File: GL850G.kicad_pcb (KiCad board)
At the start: 4 copper layers, 75 x 55 mm, 52 parts, among them J1 USB_A, J10 Conn_01x02_Pin, J2 USB_A, J3 USB_A, J4 USB_A, J5 USB_A, J6 Conn_01x03_Pin, J7 Conn_01x02_Pin, J8 Conn_01x02_Pin, J9 Conn_01x03_Pin, U1 GL850G, U11 AP2151WG, Y1 12MHz

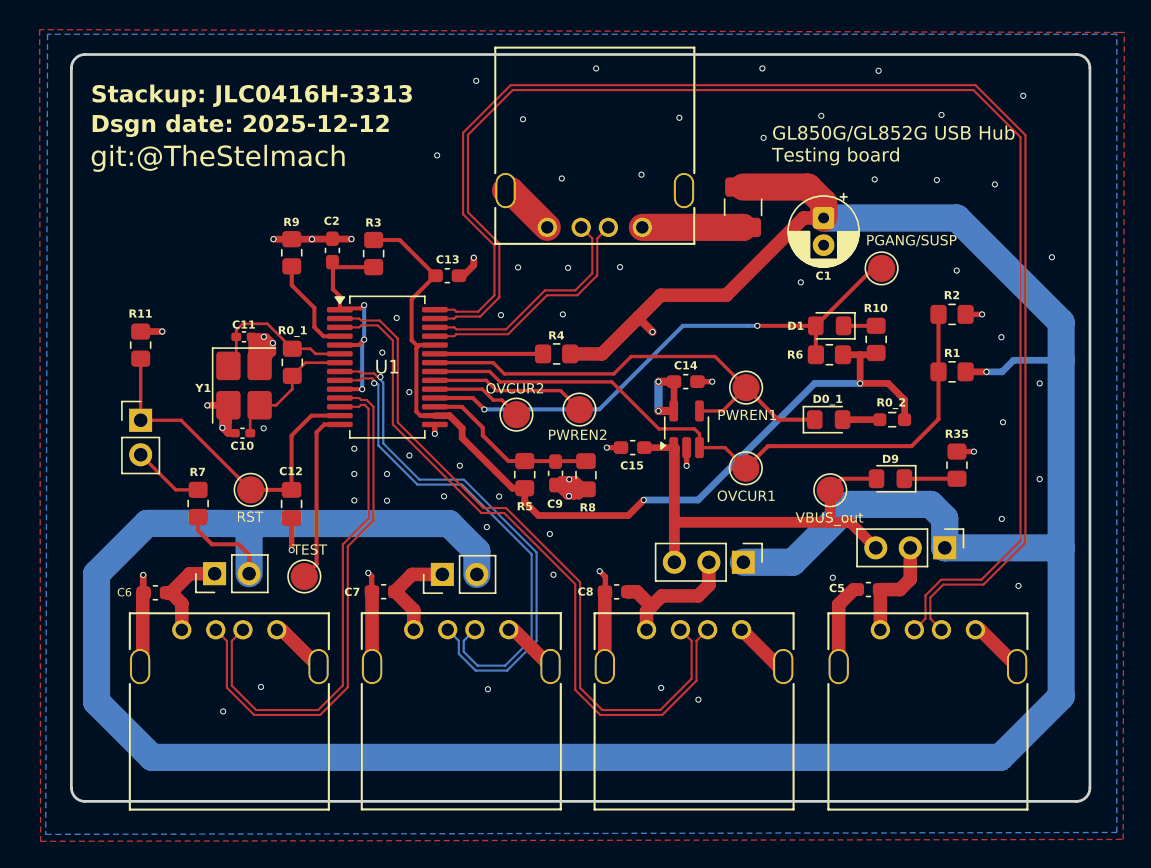
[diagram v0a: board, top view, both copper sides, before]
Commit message: modified:   0.My_Library.bak 	modified:   0.My_Library.kicad_sym 	new file:   GL850G-backups/GL850G-2026-01-02_150657.zip 	new file:   GL850G-backups/GL850G-2026-01-02_151627.zip 	new file:   GL850G-backups/GL850G-2026-01-02_160446.zip 	new file:   GL850G-backups/GL850G-2026-01-03_192335.zip 	new file:   GL850G-backups/GL850G-2026-01-03_193700.zip 	new file:   GL850G-backups/GL850G-2026-01-03_194723.zip 	new file:   GL850G-backups/GL850G-2026-01-03_195234.zip 	new file:   GL850G-backups/GL850G-2026-01-03_195824.zip 	modified:   GL850G.kicad_pcb 	modified:   GL850G.kicad_pro 	modified:   GL850G.kicad_sch 	new file:   GL850G_USB_Hub_BACKUP.zip 	modified:   fp-info-cache 	modified:   production/GL850G.zip 	new file:   production/backups/GL850G_2026-01-03_19-52-49.zip 	modified:   production/bom.csv 	modified:   production/designators.csv 	modified:   production/netlist.ipc 	modified:   production/positions.csv
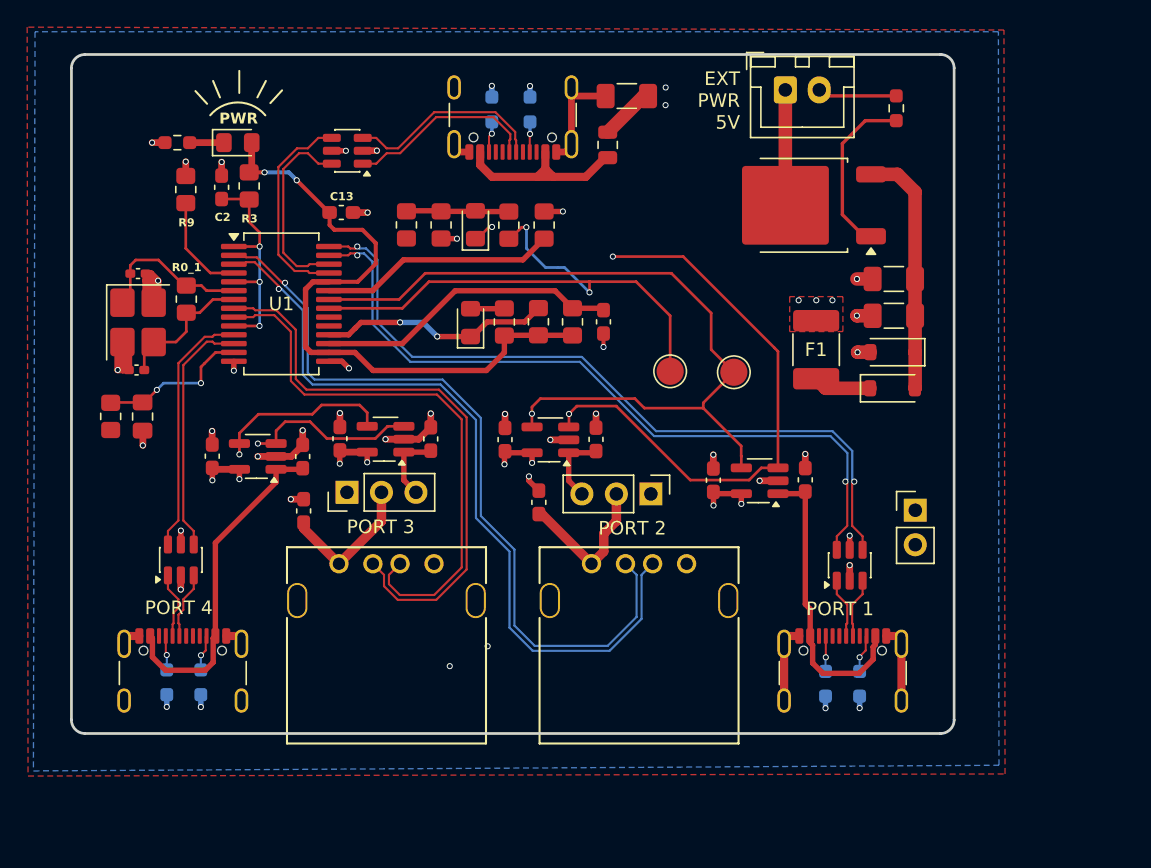
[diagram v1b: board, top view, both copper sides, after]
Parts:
- removed D9: LED, LED_SMD:LED_0805_2012Metric_Pad1.15x1.40mm_HandSolder
- removed J10, J7, J8: Conn_01x02_Pin, Connector_PinHeader_2.54mm:PinHeader_1x02_P2.54mm_Vertical
- removed J6: Conn_01x03_Pin, Connector_PinHeader_2.54mm:PinHeader_1x03_P2.54mm_Vertical
- removed R11: 100k, Resistor_SMD:R_0805_2012Metric_Pad1.20x1.40mm_HandSolder
- removed R35: 500, Resistor_SMD:R_0805_2012Metric_Pad1.20x1.40mm_HandSolder
- removed TP1, TP3, TP4, TP6, TP7, TP8: TestPoint, TestPoint:TestPoint_Pad_D2.0mm
- added C16: 2.2uF, Capacitor_SMD:C_0603_1608Metric_Pad1.08x0.95mm_HandSolder, F.Cu at (140.8, 91.8)
- added C17: 2.2uF, Capacitor_SMD:C_0603_1608Metric_Pad1.08x0.95mm_HandSolder, F.Cu at (134.1, 91.8)
- added C18: 2.2uF, Capacitor_SMD:C_0603_1608Metric_Pad1.08x0.95mm_HandSolder, F.Cu at (131.3, 93.1)
- added C19: 2.2uF, Capacitor_SMD:C_0603_1608Metric_Pad1.08x0.95mm_HandSolder, F.Cu at (124.7, 93.1)
- added C3: 2.2uF, Capacitor_SMD:C_0603_1608Metric_Pad1.08x0.95mm_HandSolder, F.Cu at (152.9, 91.8)
- added C4: 2.2uF, Capacitor_SMD:C_0603_1608Metric_Pad1.08x0.95mm_HandSolder, F.Cu at (146.2, 91.9)
- added D2: LED, LED_SMD:LED_0805_2012Metric_Pad1.15x1.40mm_HandSolder, F.Cu at (144.1, 76.0)
- added D7: BZT52C5V6, Diode_SMD:D_SOD-123, F.Cu at (174.8, 85.4)
- added D8: B5819W, Diode_SMD:D_SOD-123, F.Cu at (174.8, 88.1)
- added F4: 500mA, Fuse:Fuse_0805_2012Metric, F.Cu at (153.8, 70.2)
- added Q1: 40p04, Package_TO_SOT_SMD:TO-252-2, F.Cu at (168.1, 74.6)
- added R13: 5.1k_1%, Resistor_SMD:R_0603_1608Metric_Pad0.98x0.95mm_HandSolder, B.Cu at (172.3, 109.8)
- added R14: 5.1k_1%, Resistor_SMD:R_0603_1608Metric_Pad0.98x0.95mm_HandSolder, B.Cu at (169.8, 109.8)
- added R15: 5.1k_1%, Resistor_SMD:R_0603_1608Metric_Pad0.98x0.95mm_HandSolder, B.Cu at (123.8, 109.7)
- added R16: 5.1k_1%, Resistor_SMD:R_0603_1608Metric_Pad0.98x0.95mm_HandSolder, B.Cu at (121.3, 109.7)
- added R26: 10k, Resistor_SMD:R_0603_1608Metric_Pad0.98x0.95mm_HandSolder, F.Cu at (175.0, 67.5)
- added R67: 5.1k_1%, Resistor_SMD:R_0603_1608Metric_Pad0.98x0.95mm_HandSolder, B.Cu at (145.3, 67.5)
- added R68: 5.1k_1%, Resistor_SMD:R_0603_1608Metric_Pad0.98x0.95mm_HandSolder, B.Cu at (148.1, 67.5)
- added U12: USBLC6-2SC6, Package_TO_SOT_SMD:SOT-23-6, F.Cu at (134.6, 70.6)
- added U2: AP2141WG, Package_TO_SOT_SMD:SOT-23-5_HandSoldering, F.Cu at (149.6, 91.9)
- added U3: AP2141WG, Package_TO_SOT_SMD:SOT-23-5_HandSoldering, F.Cu at (137.4, 91.8)
- added U4: AP2141WG, Package_TO_SOT_SMD:SOT-23-5_HandSoldering, F.Cu at (128.0, 93.1)
- added U5: USBLC6-2SC6, Package_TO_SOT_SMD:SOT-23-6, F.Cu at (171.6, 101.1)
- added U6: USBLC6-2SC6, Package_TO_SOT_SMD:SOT-23-6, F.Cu at (122.4, 100.7)
- added USB1: USB_C_Recep._USB2.0_16P, Connector_USB:USB_C_Receptacle_GCT_USB4105-xx-A_16P_TopMnt_Horizontal, F.Cu at (146.8, 67.0)
- added USB2: USB_C_Recep._USB2.0_16P, Connector_USB:USB_C_Receptacle_GCT_USB4105-xx-A_16P_TopMnt_Horizontal, F.Cu at (171.1, 110.0)
- added USB3: USB_C_Recep._USB2.0_16P, Connector_USB:USB_C_Receptacle_GCT_USB4105-xx-A_16P_TopMnt_Horizontal, F.Cu at (122.5, 110.0)
- C1: footprint Capacitor_THT:CP_Radial_D5.0mm_P2.00mm -> Capacitor_SMD:C_1206_3216Metric_Pad1.33x1.80mm_HandSolder
- C5, C6: value 100nF -> 100uF; footprint Capacitor_SMD:C_0603_1608Metric_Pad1.08x0.95mm_HandSolder -> Capacitor_SMD:C_1206_3216Metric_Pad1.33x1.80mm_HandSolder
- F1: value Fuse_Small -> Fuse; footprint Fuse:Fuse_1210_3225Metric_Pad1.42x2.65mm_HandSolder -> Capacitor_SMD:C_1812_4532Metric_Pad1.57x3.40mm_HandSolder
- J1: value USB_A -> Conn_01x03_Pin; footprint My_Library:USB_A_2.0 -> Connector_PinHeader_2.54mm:PinHeader_1x03_P2.54mm_Vertical
- J2: value USB_A -> 5V; footprint My_Library:USB_A_2.0 -> Connector_JST:JST_XH_B2B-XH-A_1x02_P2.50mm_Vertical
- J3: value USB_A -> 5V_OUT; footprint My_Library:USB_A_2.0 -> Connector_PinHeader_2.54mm:PinHeader_1x02_P2.54mm_Vertical
- R0_2: value 100k -> 1k
- R1: value 10k -> 1k
- R10: value 1k -> 2k
- R2: value 20k -> 2k
- R8: value ? -> 1k; footprint Capacitor_SMD:C_0805_2012Metric_Pad1.18x1.45mm_HandSolder -> Resistor_SMD:R_0805_2012Metric_Pad1.20x1.40mm_HandSolder
- U1: value GL850G -> GL850G/GL852G
- U11: value AP2151WG -> AP2141WG
- moved C6 59.1 mm to (174.9, 80.0)
- moved R0_2 56.5 mm to (122.1, 70.0)
- moved J3 51.3 mm to (176.4, 97.1)
- moved D0_1 48.1 mm to (126.6, 70.0)
- moved R1 41.6 mm to (139.0, 76.0), turned to -90 degrees
- moved J2 41.1 mm to (166.9, 66.1)
- moved R2 38.2 mm to (141.5, 76.1), turned to 90 degrees
- moved R10 27.4 mm to (146.2, 83.2), turned to 90 degrees
- moved J1 26.7 mm to (134.6, 95.7), turned to 90 degrees
- moved D1 26.4 mm to (143.7, 83.2), turned to 90 degrees
- moved R6 21.6 mm to (148.7, 83.2), turned to 90 degrees
- moved C5 20.2 mm to (174.9, 82.7), turned to 180 degrees
- moved R8 19.3 mm to (146.5, 76.1), turned to 90 degrees
- moved C1 17.0 mm to (155.2, 66.6), turned to 180 degrees
- moved C15 12.9 mm to (168.3, 94.8), turned to 90 degrees
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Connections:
- C15 pad 1: VBUS_out -> VBUS_out1
- C5 pad 1: Net-(J2-VBUS) -> Net-(D7-K)
- C6 pad 1: Net-(J3-VBUS) -> Net-(D7-K)
- C7 pad 1: Net-(J4-VBUS) -> Net-(J1-Pin_2)
- D0_1 pad 1: /PWREN1 -> Net-(D0_1-K)
- D0_1 pad 2: Net-(D0_1-A) -> +3V3
- D1 pad 1: Net-(D1-K) -> /PGANG/SUSP
- D1 pad 2: /PGANG/SUSP -> Net-(D1-A)
- F1 pad 1: Net-(J1-VBUS) -> Net-(D8-K)
- J1 pad 1: Net-(J1-VBUS) -> +5V
- J1 pad 2: /D0N -> Net-(J1-Pin_2)
- J1 pad 3: /D0P -> VBUS_out3
- J2 pad 1: Net-(J2-VBUS) -> Net-(J2-Pin_1)
- J2 pad 2: /D1N -> GND
- J3 pad 1: Net-(J3-VBUS) -> +5V
- J3 pad 2: /D4N -> GND
- J4 pad 1: Net-(J4-VBUS) -> Net-(J1-Pin_2)
- J9 pad 3: VBUS_out -> VBUS_out2
- R0_2 pad 1: +3V3 -> Net-(D0_1-K)
- R0_2 pad 2: Net-(D0_1-A) -> GND
- R1 pad 1: /OVCUR1 -> Net-(D2-A)
- R10 pad 1: Net-(D1-K) -> +3V3
- R10 pad 2: +3V3 -> Net-(D1-A)
- R2 pad 2: /OVCUR1 -> Net-(D2-A)
- R7 pad 2: Net-(J10-Pin_2) -> /RST
- R8 pad 1: 3V -> /OVCUR1
- R8 pad 2: GND -> Net-(D2-A)
- TP2 pad 1: VBUS_out -> /PWREN1
- U1 pad 14: Net-(U1-TEST/SCL) -> GND
- U1 pad 19: /OVCUR2 -> unconnected-(U1-OVCUR2-Pad19)
- U1 pad 20: /PWREN2 -> unconnected-(U1-PWREN2-Pad20)
- U11 pad 1: VBUS_out -> VBUS_out1
- U11 pad 3: /OVCUR1 -> /OVCUR_FLG
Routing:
- net +5V: track 252.0 -> 23.7 mm, vias 4 -> 17
- net /OVCUR_FLG: track 0.00 -> 113.6 mm, vias 0 -> 5
- net /PWREN1: track 34.9 -> 121.1 mm, vias 0 -> 3
- net /D1N: track 103.1 -> 54.7 mm, vias 0 -> 2
- net /D1P: track 103.7 -> 55.3 mm, vias 0 -> 2
- net VBUS_out: track 32.3 -> 0.00 mm
- net VBUS_out4: track 0.00 -> 24.9 mm
- net /PGANG/SUSP: track 39.7 -> 17.1 mm
- net VBUS_out1: track 0.00 -> 21.9 mm
- net /D4N: track 39.4 -> 18.6 mm
- net +3V3: track 68.6 -> 48.2 mm
- net /D4P: track 37.6 -> 18.0 mm
- net Net-(D7-K): track 0.00 -> 18.2 mm
- net /D0_P: track 0.00 -> 14.8 mm
- net /RST: track 25.9 -> 11.3 mm, vias 0 -> 2
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- added copper zone on B.Cu, net +5V
- added copper zone on F.Cu, net +5V
- removed copper zone on B.Cu, net GND
- removed copper zone on F.Cu, net GND
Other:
- board size 75 x 55 mm -> 65 x 50 mm
- board text added: "Dsgn date: 2026-01-03"
- board text added: "EXT PWR 5V"
- board text added: "GL850G/GL852G USB Hub V1.1"
- board text added: "PORT 1"
- board text added: "PORT 2"
- board text added: "PORT 3"
- board text added: "PORT 4"
- board text added: "PWR"
- board text removed: "Dsgn date: 2025-12-12"
- board text removed: "GL850G/GL852G USB Hub Testing board"
- board text removed: "OVCUR1"
- board text removed: "OVCUR2"
- board text removed: "PGANG/SUSP"
- board text removed: "PWREN1"
- board text removed: "PWREN2"
- board text removed: "RST"
- board text removed: "TEST"
- board text removed: "VBUS_out"
